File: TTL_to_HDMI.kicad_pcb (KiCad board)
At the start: 4 copper layers, 59 x 47 mm, 68 parts, among them J1 HDMI_A_1.4, J2 Conn_01x19_Female, J3 Conn_01x19_Female, U1 1x50, U2 1x50, U3 TFP410PAP, U4 MT3420C

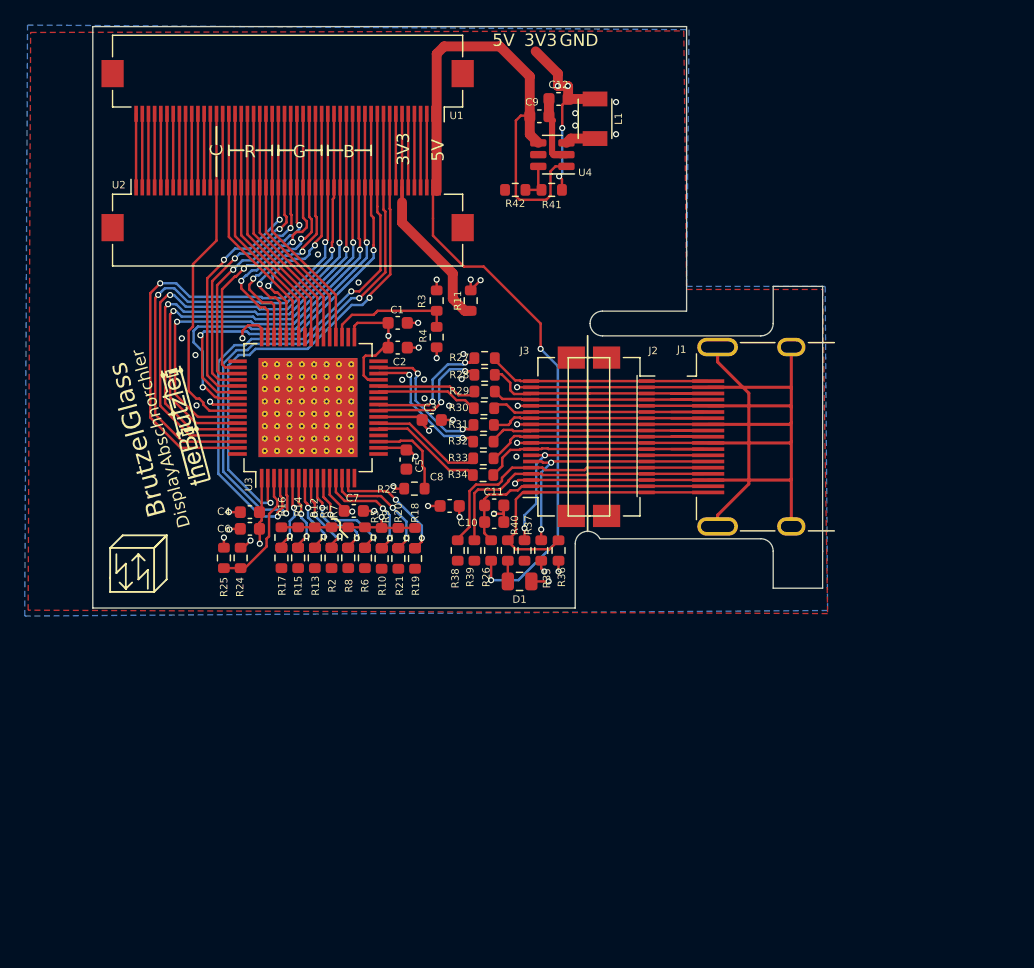
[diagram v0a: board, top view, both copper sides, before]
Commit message: Upload_V3 V4 and PDF V3
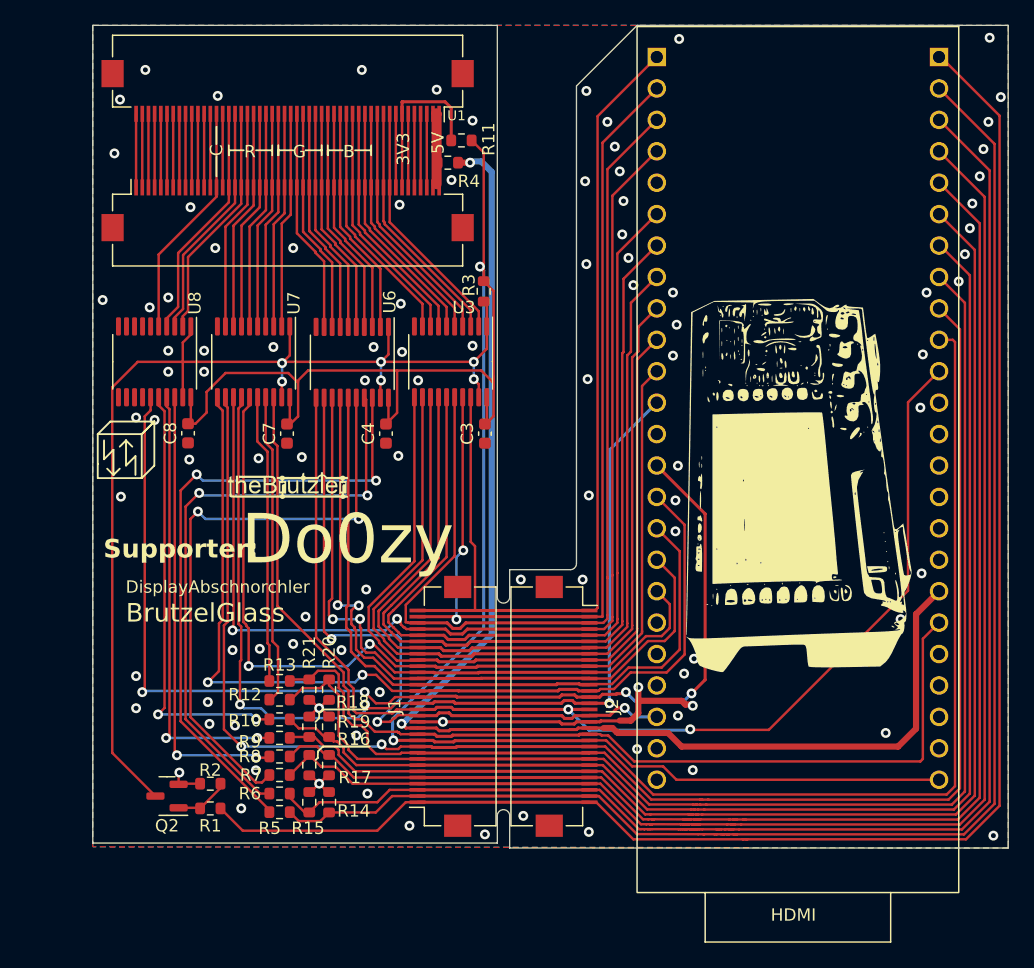
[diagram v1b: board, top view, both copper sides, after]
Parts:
- removed C1, C10, C12, C5, C6, C9: 4µ7, Capacitor_SMD:C_0603_1608Metric
- removed C11, C2: 100n, Capacitor_SMD:C_0603_1608Metric
- removed D1: LED, Capacitor_SMD:C_0805_2012Metric
- removed J3: Conn_01x19_Female, Connector_FFC-FPC:Hirose_FH12-19S-0.5SH_1x19-1MP_P0.50mm_Horizontal
- removed L1: 2µ2, Inductor_SMD:L_TDK_NLV32_3.2x2.5mm
- removed R22: 510, Resistor_SMD:R_0603_1608Metric
- removed R24, R25, R35, R37, R38, R39, R40: 5K, Resistor_SMD:R_0603_1608Metric
- removed R26: 0, Resistor_SMD:R_0603_1608Metric
- removed R27, R28, R29, R30, R31, R32, R33, R34: 10, Resistor_SMD:R_0603_1608Metric
- removed R36: 10K, Resistor_SMD:R_0603_1608Metric
- removed R41: 450K, Resistor_SMD:R_0603_1608Metric
- removed R42: 100K, Resistor_SMD:R_0603_1608Metric
- removed U4: MT3420C, Package_TO_SOT_SMD:SOT-23-6
- added G***: LOGO, KicadLibs:DS1054Z, F.Cu at (133.0, 109.0)
- added Q2: Q_NPN_BEC, Package_TO_SOT_SMD:SOT-23, F.Cu at (82.0, 134.2)
- added U5: NANO_9K, TheBrutzlers_Lib:Nano 9K, F.Cu at (133.0, 77.0)
- added U6: 74LVX541, Package_SO:TSSOP-20_4.4x6.5mm_P0.65mm, F.Cu at (97.0, 99.1)
- added U7: 74LVX541, Package_SO:TSSOP-20_4.4x6.5mm_P0.65mm, F.Cu at (89.0, 99.1)
- added U8: 74LVX541, Package_SO:TSSOP-20_4.4x6.5mm_P0.65mm, F.Cu at (81.0, 99.1)
- J1: value HDMI_A_1.4 -> Conn_01x32_Pin; footprint Connector_HDMI:HDMI_A_Molex_208658-1001_Horizontal -> Connector_FFC-FPC:Hirose_FH12-32S-0.5SH_1x32-1MP_P0.50mm_Horizontal
- J2: value Conn_01x19_Female -> Conn_01x32_Pin; footprint Connector_FFC-FPC:Hirose_FH12-19S-0.5SH_1x19-1MP_P0.50mm_Horizontal -> Connector_FFC-FPC:Hirose_FH12-32S-0.5SH_1x32-1MP_P0.50mm_Horizontal
- R1, R10, R12, R13, R14, R15, R16, R17, R18, R19, R20, R21, R3, R5, R6, R7, R8, R9: value 5K -> 10K
- R2: value 5K -> 100K
- R4: value 5K -> 0
- U3: value TFP410PAP -> 74LVX541; footprint Package_QFP:HTQFP-64-1EP_10x10mm_P0.5mm_EP8x8mm_Mask4.4x4.4mm_ThermalVias -> Package_SO:TSSOP-20_4.4x6.5mm_P0.65mm
- moved G*** 53.3 mm to (133.9, 83.2), turned to -90 degrees
- moved G*** 44.4 mm to (118.2, 109.4), turned to -90 degrees
- moved G*** 34.1 mm to (133.0, 109.3), turned to -90 degrees
- moved J1 33.1 mm to (104.1, 127.0), turned to 90 degrees
- moved G*** 27.5 mm to (133.8, 132.8)
- moved R1 24.0 mm to (85.5, 135.2), turned to 0 degrees
- moved R5 23.2 mm to (91.1, 135.5), turned to 0 degrees
- moved J2 22.3 mm to (114.3, 127.0)
- moved C8 22.0 mm to (83.7, 104.9), turned to 90 degrees
- moved R14 21.5 mm to (95.1, 134.7)
- moved R2 20.7 mm to (85.5, 133.2), turned to 180 degrees
- moved R6 20.3 mm to (91.1, 134.0), turned to 0 degrees
- moved R7 20.0 mm to (91.1, 132.5), turned to 0 degrees
- moved R15 19.8 mm to (93.5, 134.7)
- moved R16 18.5 mm to (93.5, 131.7), turned to 90 degrees
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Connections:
- net Net-(U1-Pad11) renamed HS
- net Net-(U1-Pad9) renamed DE
- J1 pad 1: /D2+ -> /32
- J1 pad 10: /CK+ -> F_R4
- J1 pad 11: GND -> +3V3
- J1 pad 12: /CK- -> F_G2
- J1 pad 13: /13 -> +5V
- J1 pad 14: /14 -> GND
- J1 pad 15: /15 -> F_G4
- J1 pad 16: /16 -> F_G3
- J1 pad 17: GND -> F_R6
- J1 pad 18: +5VD -> F_CLK
- J1 pad 19: /19 -> F_R3
- J1 pad 2: GND -> /31
- J1 pad 3: /D2- -> /30
- J1 pad 4: /D1+ -> /29
- J1 pad 5: GND -> /28
- J1 pad 6: /D1- -> /27
- J1 pad 7: /D0+ -> /26
- J1 pad 8: GND -> /25
- J1 pad 9: /D0- -> /24
- J2 pad 1: /D2+ -> F_DE
- J2 pad 10: /CK+ -> F_R7
- J2 pad 11: GND -> F_G5
- J2 pad 12: /CK- -> F_G6
- J2 pad 13: /13 -> F_G7
- J2 pad 14: /14 -> F_R3
- J2 pad 15: /15 -> F_CLK
- J2 pad 16: /16 -> F_R6
- J2 pad 17: GND -> F_G3
- J2 pad 18: +5VD -> F_G4
- J2 pad 19: /19 -> GND
- J2 pad 2: GND -> F_VS
- J2 pad 3: /D2- -> F_HS
- J2 pad 4: /D1+ -> F_R5
- J2 pad 5: GND -> F_B7
- J2 pad 6: /D1- -> F_B6
- J2 pad 7: /D0+ -> F_B5
- J2 pad 8: GND -> F_B4
- J2 pad 9: /D0- -> F_B3
- R1 pad 1: +3V3 -> Net-(Q2-B)
- R1 pad 2: EDGE -> /32
- R10 pad 1: nRST -> F_R0
- R10 pad 2: GND -> /26
- R12 pad 1: +3V3 -> F_G1
- R12 pad 2: CTL1 -> /25
- R13 pad 1: CTL1 -> F_G0
- R13 pad 2: GND -> /24
- R14 pad 1: +3V3 -> GND
- R14 pad 2: CTL2 -> /31
- R15 pad 1: CTL2 -> GND
- R15 pad 2: GND -> /30
- R16 pad 1: +3V3 -> GND
- R16 pad 2: CTL3 -> /29
- R17 pad 1: CTL3 -> GND
- R17 pad 2: GND -> /28
- R18 pad 1: +3V3 -> GND
- R18 pad 2: SCL -> /27
- R19 pad 1: SCL -> GND
- R19 pad 2: GND -> /26
- R2 pad 1: EDGE -> Net-(Q2-B)
- R20 pad 1: +3V3 -> GND
- R20 pad 2: SDA -> /25
- R21 pad 1: SDA -> GND
- R21 pad 2: GND -> /24
- R3 pad 2: DKEN -> F_OE1
- R4 pad 1: DKEN -> Net-(R4-Pad1)
- R4 pad 2: GND -> +5V
- R5 pad 1: +3V3 -> F_B2
- R5 pad 2: MSEN -> /31
- R6 pad 1: MSEN -> F_B1
- R6 pad 2: GND -> /30
- R7 pad 1: +3V3 -> F_B0
- R7 pad 2: nPD -> /29
- R8 pad 1: nPD -> F_R2
- R8 pad 2: GND -> /28
- R9 pad 1: +3V3 -> F_R1
- R9 pad 2: nRST -> /27
- U1 pad 1: +5V -> Net-(R4-Pad1)
- U1 pad 10: Net-(U1-Pad10) -> VS
- U1 pad 2: +5V -> Net-(R4-Pad1)
- U2 pad 41: Net-(U1-Pad10) -> VS
- U2 pad 49: +5V -> Net-(R4-Pad1)
- U2 pad 50: +5V -> Net-(R4-Pad1)
- U3 pad 1: +3V3 -> F_OE1
- U3 pad 10: nPD -> GND
- U3 pad 11: MSEN -> F_B3
- U3 pad 12: +3V3 -> F_B4
- U3 pad 13: nRST -> F_B5
- U3 pad 14: SDA -> F_B6
- U3 pad 15: SCL -> F_B7
- U3 pad 16: GND -> F_HS
- U3 pad 17: GND -> F_VS
- U3 pad 18: +3V3 -> F_DE
- U3 pad 19: Net-(R22-Pad1) -> F_OE1
- U3 pad 20: GND -> +3V3
- U3 pad 3: Net-(U3-Pad3) -> VS
- U3 pad 5: Net-(U1-Pad10) -> B7
- U3 pad 6: CTL3 -> B6
- U3 pad 7: CTL2 -> B5
- U3 pad 8: CTL1 -> B4
- U3 pad 9: EDGE -> B3
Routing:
- net GND: track 192.4 -> 60.1 mm, vias 37 -> 101
- net /32: track 0.00 -> 129.7 mm
- net F_R4: track 0.00 -> 126.2 mm, vias 0 -> 2
- net /31: track 0.00 -> 120.1 mm
- net /30: track 0.00 -> 117.2 mm
- net /29: track 0.00 -> 114.0 mm
- net /28: track 0.00 -> 110.4 mm
- net /27: track 0.00 -> 107.1 mm
- net /25: track 0.00 -> 104.9 mm
- net /26: track 0.00 -> 104.1 mm
- net /24: track 0.00 -> 101.2 mm
- net F_G3: track 0.00 -> 99.3 mm, vias 0 -> 2
- net +3V3: track 60.4 -> 158.3 mm, vias 15 -> 2
- net F_OE1: track 0.00 -> 91.0 mm, vias 0 -> 6
- net F_CLK: track 0.00 -> 90.6 mm, vias 0 -> 4
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- added copper zone on B.Cu, net GND
- removed copper zone on B.Cu, net +3V3
- removed copper zone on In1.Cu, net GND
- removed copper zone on In2.Cu, net GND
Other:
- board size 59 x 47 mm -> 74 x 66.5 mm
- copper layers 4 -> 2
- board text added: "Do0zy"
- board text added: "Supporter:"
- board text removed: "GND"
- board text removed: "this PCB is to convert TTL Display- signals to HDMI the Pinout is take´n from the TM070RDH13"
